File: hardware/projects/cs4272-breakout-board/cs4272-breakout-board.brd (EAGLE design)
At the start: 20 parts, among them Q1 24.576M, U1 CS4272

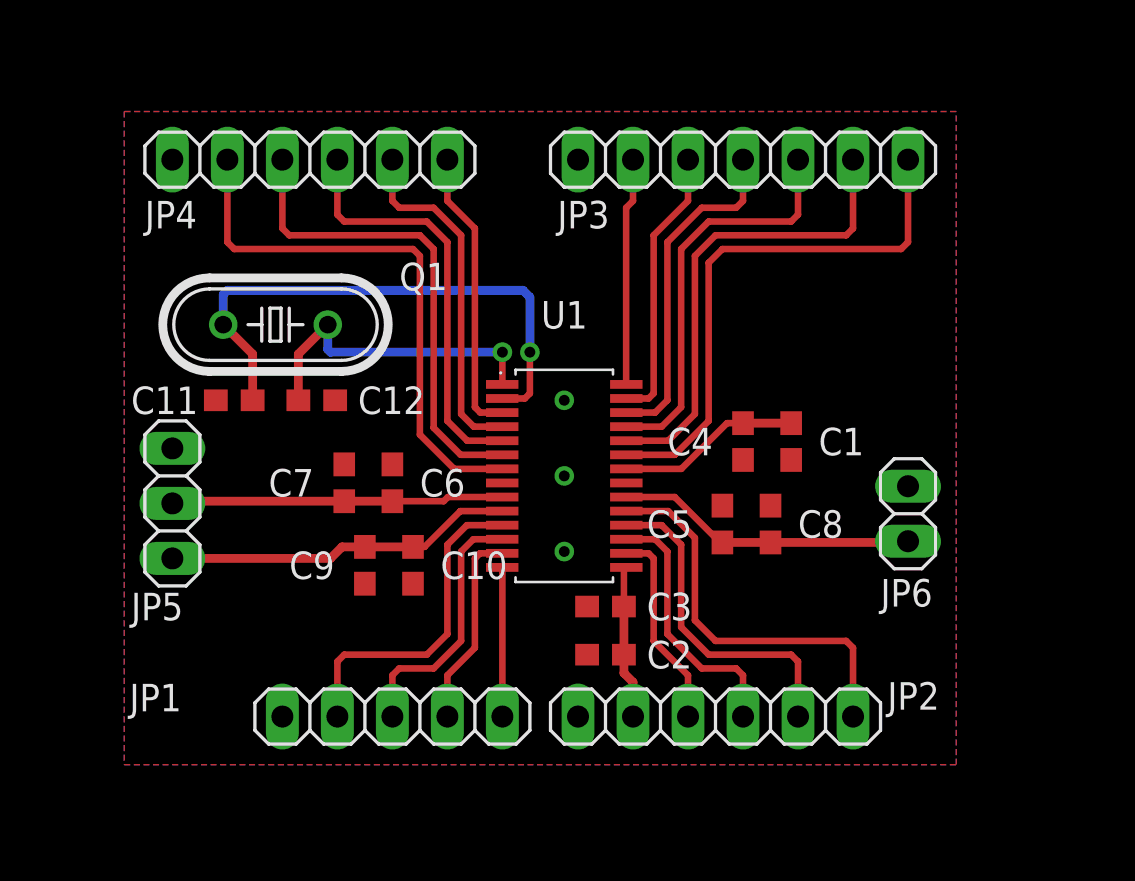
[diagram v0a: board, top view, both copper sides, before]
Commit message: Update breakout board
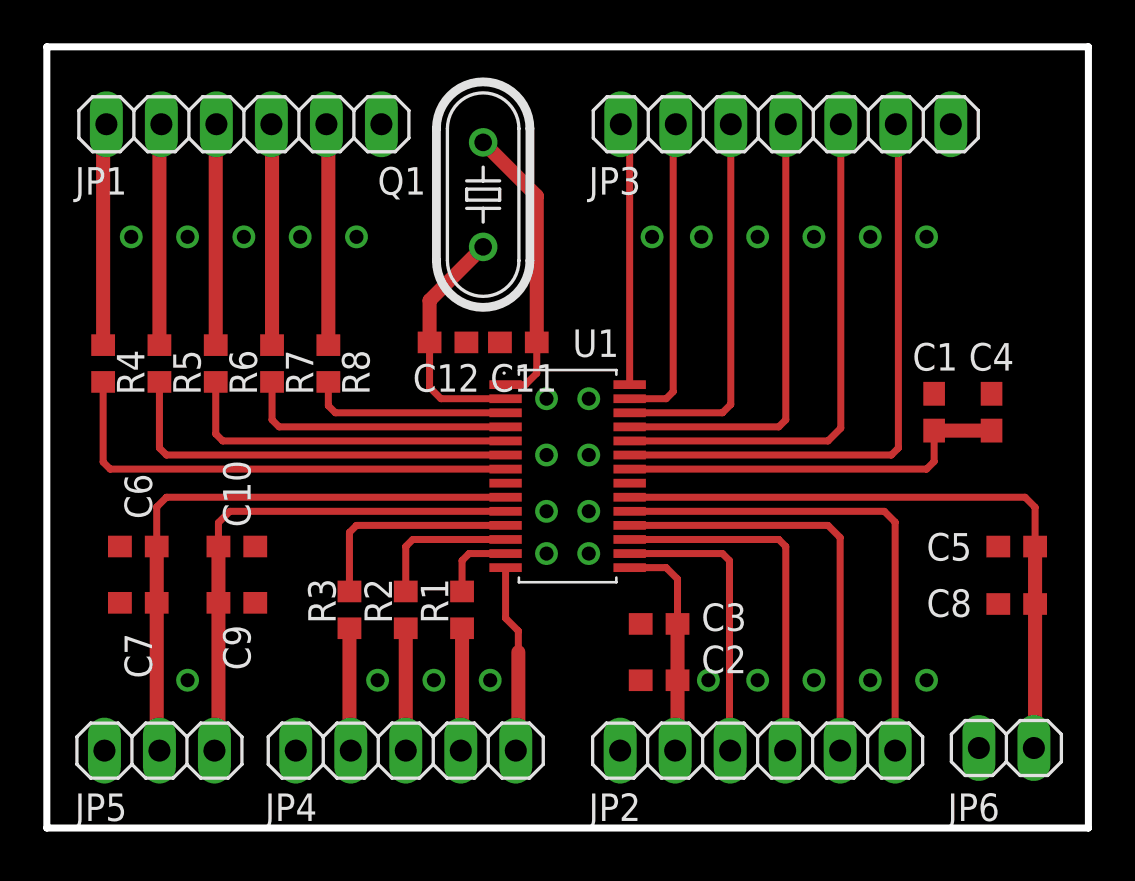
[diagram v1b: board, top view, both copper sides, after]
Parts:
- added R1, R2, R3, R4, R5, R6, R7, R8: (no value), rcl:R0603
- JP1: value I2C/SPI -> I2S; device pinhead:1X05 -> pinhead:1X06
- JP4: value I2S -> I2C/SPI; device pinhead:1X06 -> pinhead:1X05
- moved JP1 28.2 mm to (5.53, 29.6), turned to 180 degrees
- moved JP4 27.6 mm to (13.0, 0.65), turned to 0 degrees
- moved C5 13.6 mm to (41.2, 10.1), turned to 180 degrees
- moved C6 12.1 mm to (0.65, 10.1), turned to 0 degrees
- moved C8 12.0 mm to (41.2, 7.42), turned to 180 degrees
- moved JP6 11.7 mm to (40.7, 0.77), turned to 0 degrees
- moved JP5 11.4 mm to (1.62, 0.65), turned to 0 degrees
- moved Q1 11.3 mm to (16.6, 26.3), turned to 270 degrees
- moved C7 11.0 mm to (0.65, 7.47), turned to 0 degrees
- moved C11 10.2 mm to (14.9, 19.5), turned to 180 degrees
- moved C12 9.69 mm to (18.2, 19.5), turned to 0 degrees
- moved C1 9.35 mm to (40.1, 16.3), turned to 90 degrees
- moved C4 8.93 mm to (37.4, 16.3), turned to 90 degrees
- moved C9 8.18 mm to (5.20, 10.1), turned to 0 degrees
- moved C10 6.16 mm to (5.20, 7.47), turned to 0 degrees
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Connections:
- new net N$1: JP4.4, R1.1
- new net N$2: JP4.3, R2.1
- new net N$3: JP4.2, R3.1
- new net N$4: JP1.2, R8.1
- new net N$5: JP1.3, R7.1
- new net N$6: JP1.4, R6.1
- new net N$7: JP1.5, R5.1
- new net N$8: JP1.6, R4.1
- net !AMUTEC!: now also JP3.2; no longer JP3.1
- net !BMUTEC!: now also JP3.7; no longer JP3.6
- net !RST!: now also JP4.5; no longer JP1.5
- net AD0/!CS!(I2S/!LJ!): now also R1.2; no longer JP1.4
- net AOUTA+: now also JP3.4; no longer JP3.3
- net AOUTA-: now also JP3.3; no longer JP3.2
- net AOUTB+: now also JP3.5; no longer JP3.4
- net AOUTB-: now also JP3.6; no longer JP3.5
- net GND: now also JP3.1, JP4.1; no longer JP3.7, JP4.6
- net LRCK: now also R7.2; no longer JP4.2
- net MCLK: now also R8.2; no longer JP4.1
- net SCL/CCLK(M0): now also R3.2; no longer JP1.2
- net SCLK: now also R6.2; no longer JP4.3
- net SDA/CDIN(M1): now also R2.2; no longer JP1.3
- net SDIN: now also R4.2; no longer JP4.5
- net SDOUT(M/!S!): now also R5.2; no longer JP4.4
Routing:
- net VA: track 13.9 -> 30.1 mm
- net XTI: track 25.6 -> 11.2 mm, vias 1 -> 0
- net VD: track 15.4 -> 27.6 mm
- net N$8: track 0.00 -> 10.3 mm
- net N$7: track 0.00 -> 10.2 mm
- net N$4: track 0.00 -> 10.2 mm
- net N$6: track 0.00 -> 10.2 mm
- net N$5: track 0.00 -> 10.2 mm
- net FILT+: track 8.49 -> 18.3 mm
- net VL: track 16.1 -> 24.1 mm
- net N$3: track 0.00 -> 5.67 mm
- net N$1: track 0.00 -> 5.67 mm
- net N$2: track 0.00 -> 5.65 mm
- net AD0/!CS!(I2S/!LJ!): track 9.19 -> 3.57 mm
- net SDA/CDIN(M1): track 12.0 -> 6.82 mm
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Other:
- board outline added: 48.1 x 36.1 mm
